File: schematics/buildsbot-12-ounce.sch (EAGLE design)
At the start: 16 parts, among them IC1 L293E, J1 1X2-3.5MM, J2 1X2-3.5MM, U1 ARDUINO_SHIELDLABEL

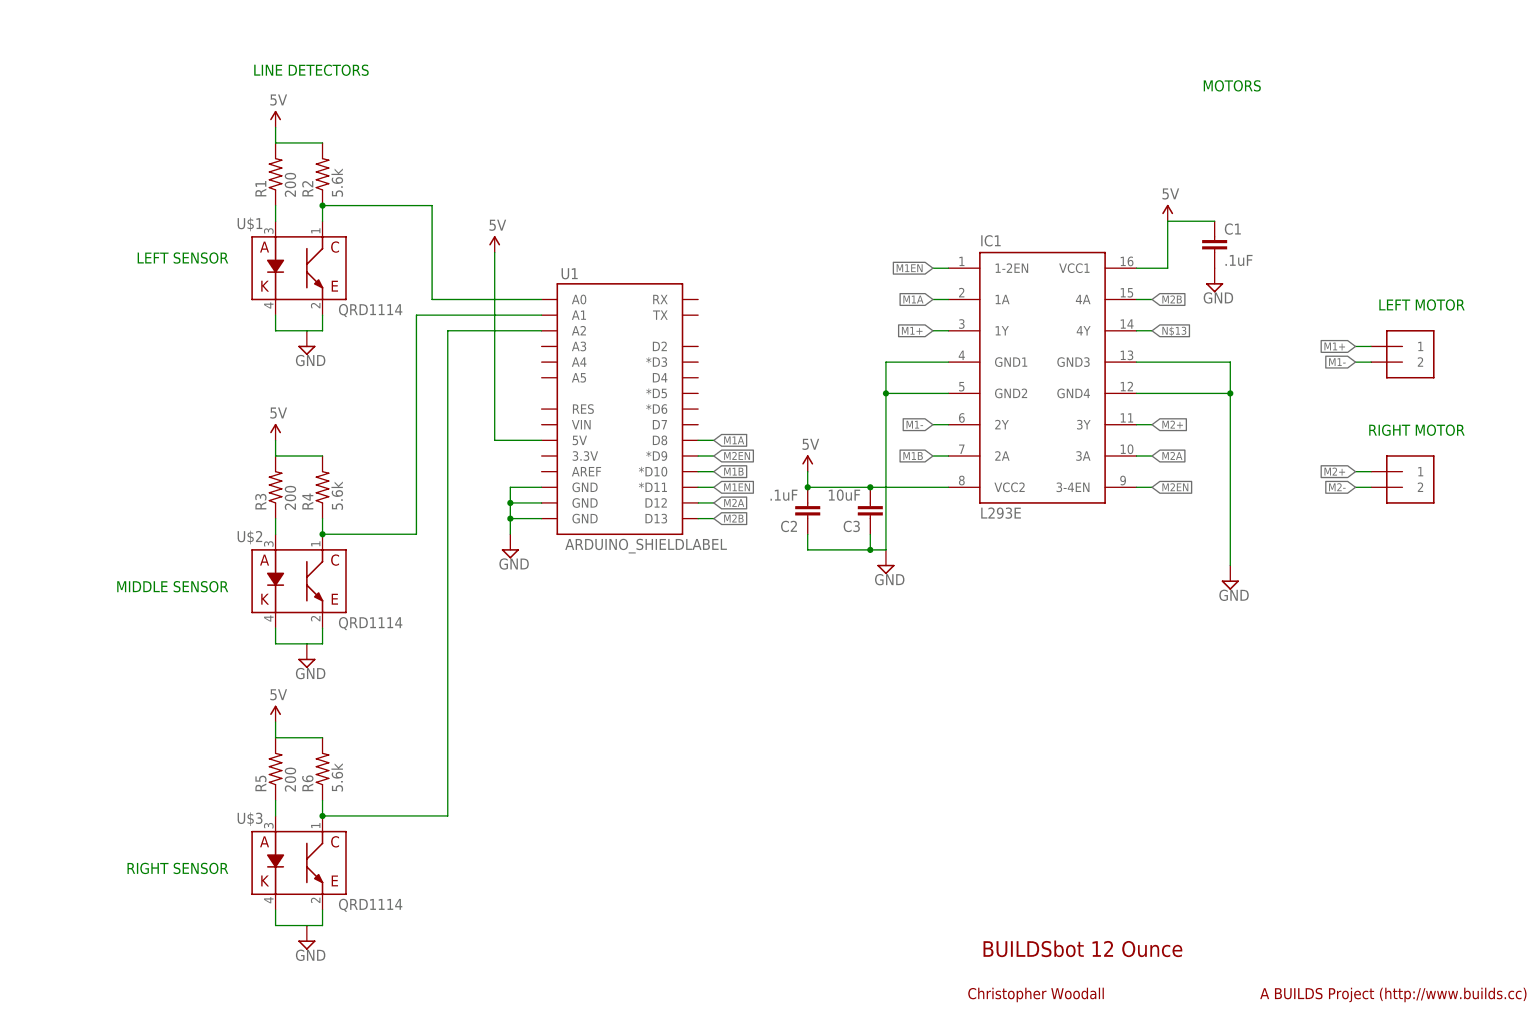
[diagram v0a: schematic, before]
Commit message: Fixing up some schematics
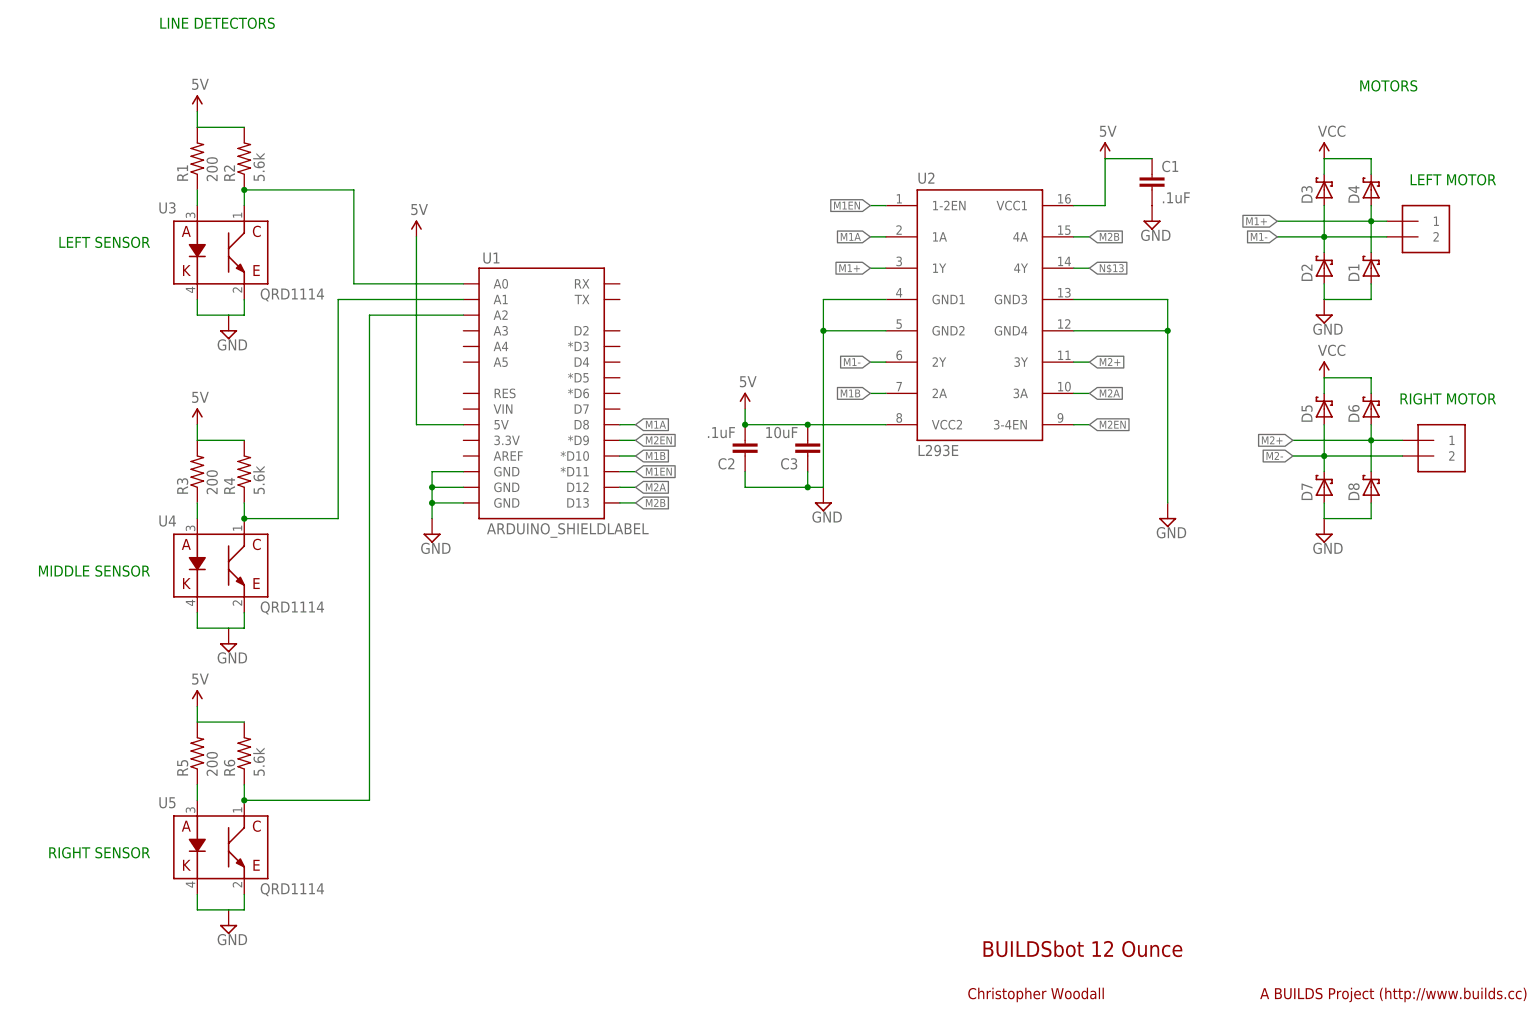
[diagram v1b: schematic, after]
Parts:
- removed IC1: L293E, texas:L293E
- removed U$1, U$2, U$3: QRD1114, SparkFun:QRD1114
- added D1, D2, D3, D4, D5, D6, D7, D8: (no value), adafruit:SCHOTTKY-DIODEC4111-15
- added U2: L293E, texas:L293E
- added U3, U4, U5: QRD1114, SparkFun:QRD1114
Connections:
- net GND: now also D1.A, D2.A, D7.A, D8.A, U3.C, U3.K, U4.C, U4.K, U5.C, U5.K; no longer U$1.C, U$1.K, U$2.C, U$2.K, U$3.C, U$3.K
- net M1+: now also D1.C, D4.A, U2.1Y; no longer IC1.1Y
- net M1-: now also D2.C, D3.A, U2.2Y; no longer IC1.2Y
- net M1A: now also U2.1A; no longer IC1.1A
- net M1B: now also U2.2A; no longer IC1.2A
- net M1EN: now also U2.1-2EN; no longer IC1.1-2EN
- net M2+: now also D6.A, D8.C, U2.3Y; no longer IC1.3Y
- net M2-: now also D5.A, D7.C, U2.GND1, U2.GND2, U2.GND3, U2.GND4; no longer IC1.GND1, IC1.GND2, IC1.GND3, IC1.GND4
- net M2A: now also U2.3A; no longer IC1.3A
- net M2B: now also U2.4A; no longer IC1.4A
- net M2EN: now also U2.3-4EN; no longer IC1.3-4EN
- net N$13: now also U2.4Y; no longer IC1.4Y
- net N$4: now also U3.E; no longer U$1.E
- net N$5: now also U3.A; no longer U$1.A
- net N$6: now also U4.E; no longer U$2.E
- net N$7: now also U4.A; no longer U$2.A
- net N$8: now also U5.E; no longer U$3.E
- net N$9: now also U5.A; no longer U$3.A
- net VCC: now also D3.C, D4.C, D5.C, D6.C, U2.VCC1, U2.VCC2; no longer IC1.VCC1, IC1.VCC2
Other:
- moved on the sheet: C1, C2, C3, R1, R2, R3, R4, R5, R6, U1
